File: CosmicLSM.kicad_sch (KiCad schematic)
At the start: 49 parts, among them J1 BAT, J2 JST GH, J3 USB_C_Receptacle_USB2.0, SW1 SW_SPDT, SW2 SW_SPST, U1 SMF05CT1G, U2 SMF05CT1G, U3 M3406, U4 IP2312, U5 LSM6DSV, U7 ESP32-C6-MINI-1/U

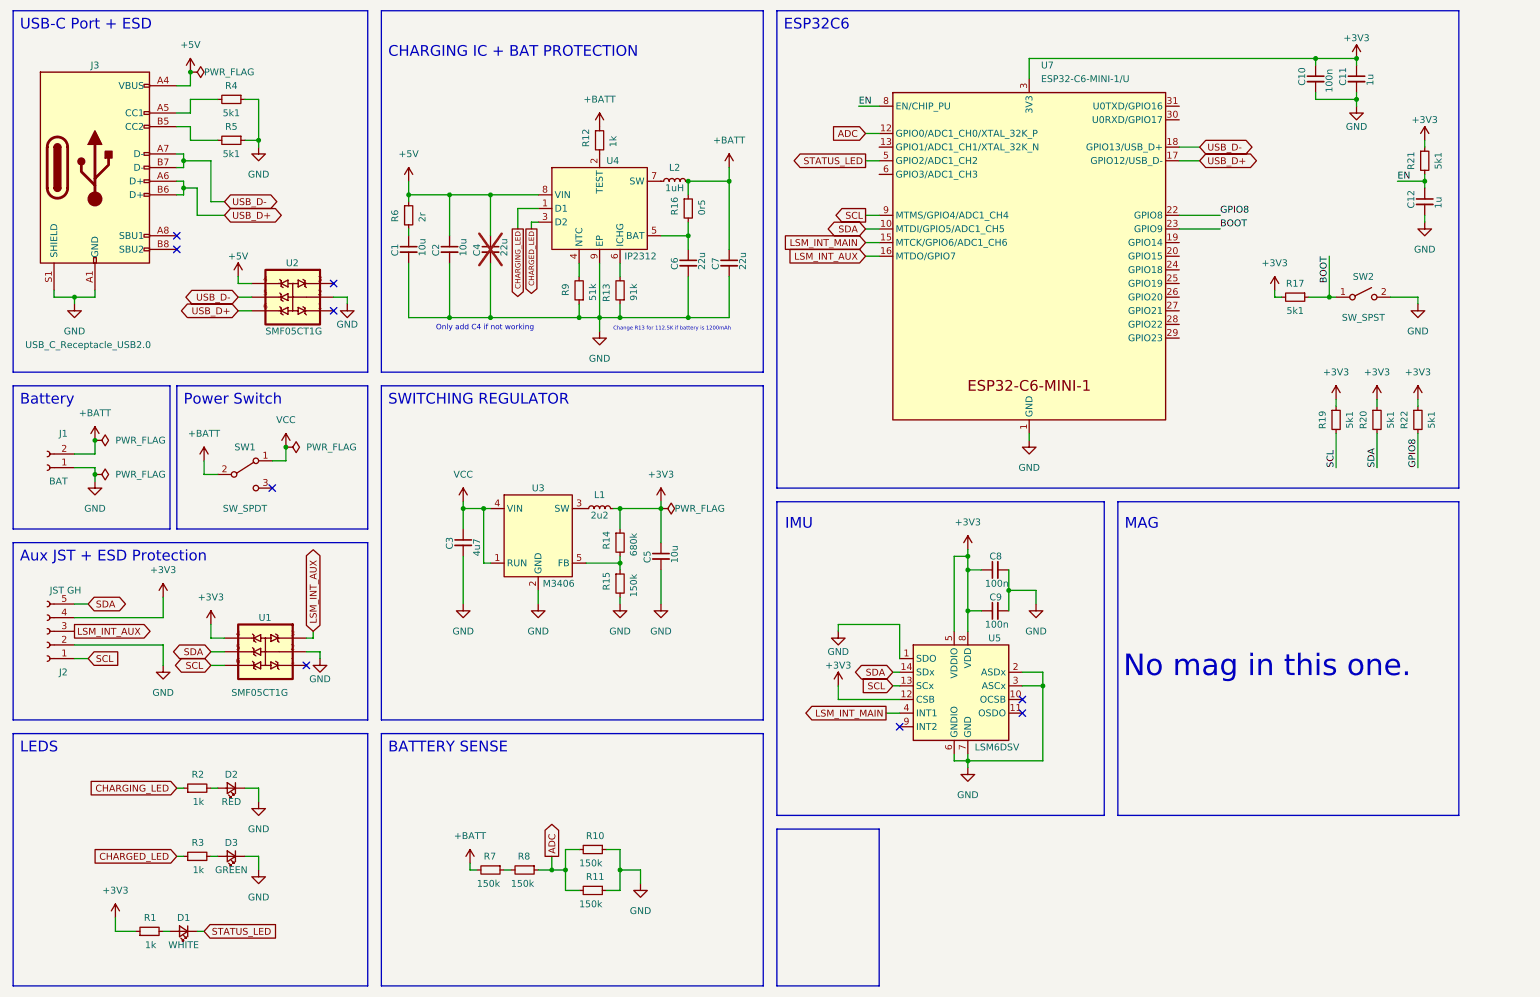
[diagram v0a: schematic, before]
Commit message: new data
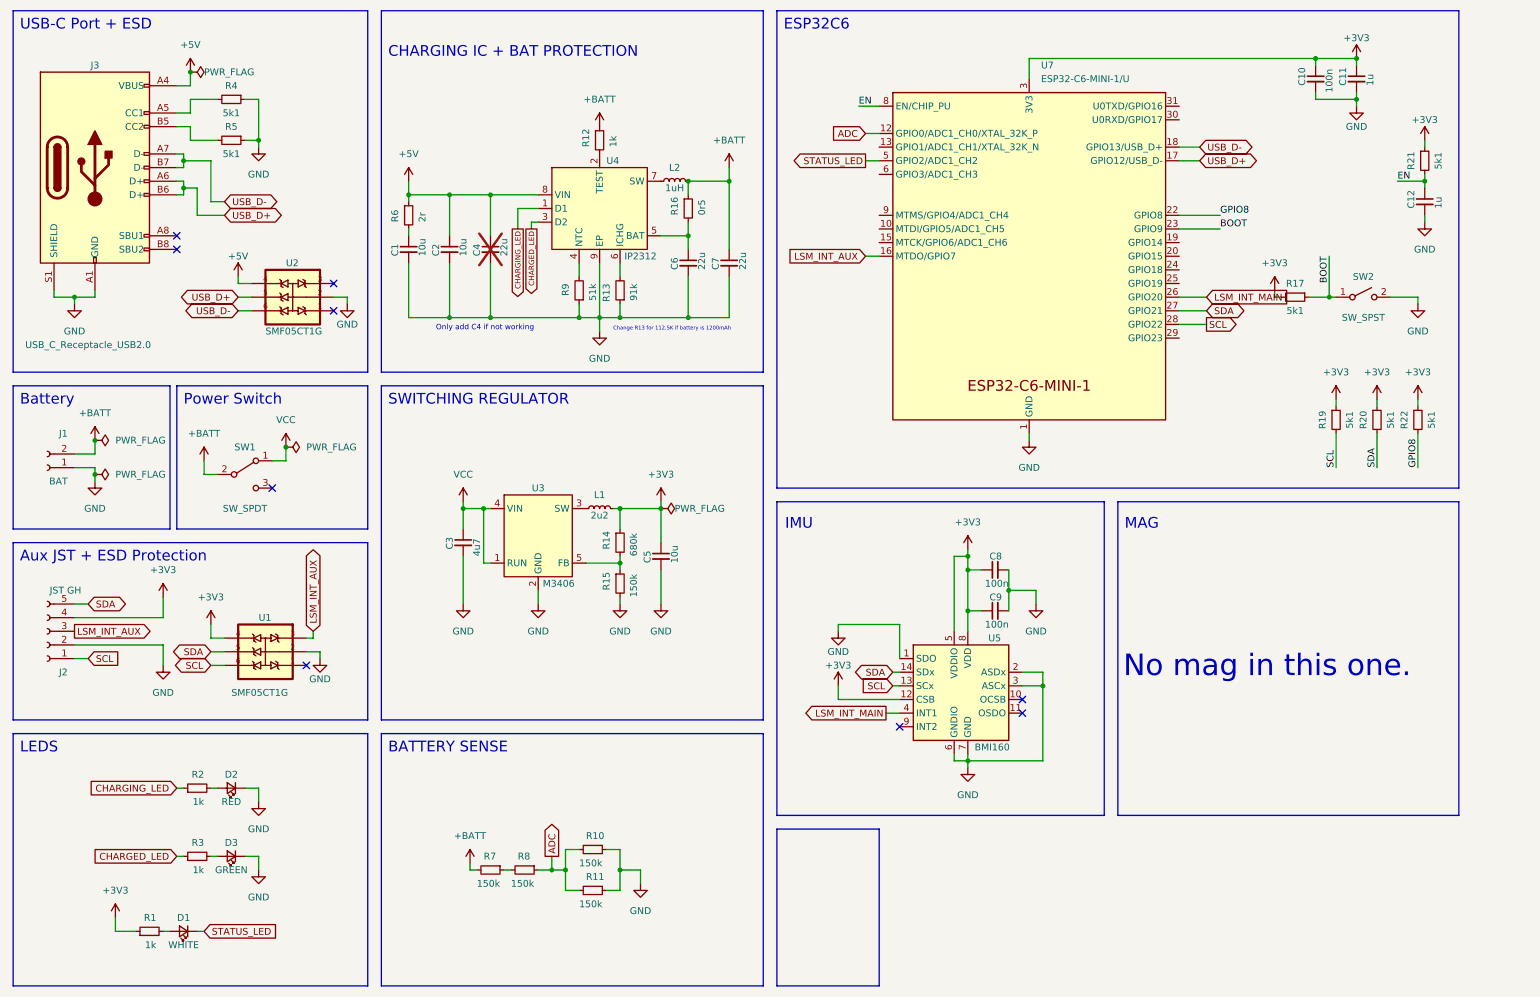
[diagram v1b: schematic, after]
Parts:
- U5: value LSM6DSV -> BMI160
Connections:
- net LSM_INT_MAIN: now also U7.26 (GPIO20); no longer U7.15 (MTCK/GPIO6/ADC1_CH6)
- net SCL: now also U7.28 (GPIO22); no longer U7.9 (MTMS/GPIO4/ADC1_CH4)
- net SDA: now also U7.27 (GPIO21); no longer U7.10 (MTDI/GPIO5/ADC1_CH5)
- net USB_D+: now also U2.5; no longer U2.6
- net USB_D-: now also U2.6; no longer U2.5
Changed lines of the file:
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@@
 	(wire
 		(pts
-			(xy 172.72 54.61) (xy 175.26 54.61)
-		)
-		(stroke
-			(width 0)
-			(type default)
-		)
-	)
-	(wire
-		(pts
 			(xy 73.66 67.31) (xy 76.2 67.31)
 		)
@@
 	(wire
 		(pts
-			(xy 45.72 41.91) (xy 45.72 40.64)
+			(xy 231.14 67.31) (xy 236.22 67.31)
 		)
 		(stroke
@@
 	(wire
 		(pts
-			(xy 172.72 57.15) (xy 175.26 57.15)
+			(xy 231.14 72.39) (xy 236.22 72.39)
+		)
+		(stroke
+			(width 0)
+			(type default)
+		)
+	)
+	(wire
+		(pts
+			(xy 45.72 41.91) (xy 45.72 40.64)
 		)
 		(stroke
@@
 	(wire
 		(pts
-			(xy 172.72 52.07) (xy 175.26 52.07)
-		)
-		(stroke
-			(width 0)
-			(type default)
-		)
-	)
-	(wire
-		(pts
 			(xy 116.84 173.99) (xy 116.84 170.18)
 		)
@@
 	(wire
 		(pts
+			(xy 231.14 69.85) (xy 236.22 69.85)
+		)
+		(stroke
+			(width 0)
+			(type default)
+		)
+	)
+	(wire
+		(pts
 			(xy 124.46 170.18) (xy 127 170.18)
 		)
@@
 		)
 	)
-	(global_label "USB_D-"
+	(global_label "USB_D+"
 		(shape bidirectional)
 		(at 55.88 67.31 180)
@@
 		)
 	)
-	(global_label "USB_D+"
+	(global_label "USB_D-"
 		(shape bidirectional)
 		(at 55.88 69.85 180)
@@
 	(global_label "SDA"
 		(shape bidirectional)
-		(at 172.72 54.61 180)
+		(at 236.22 69.85 0)
 		(fields_autoplaced yes)
 		(effects
@@
 				(size 1.27 1.27)
 			)
-			(justify right)
+			(justify left)
 		)
 		(property "Intersheetrefs" "${INTERSHEET_REFS}"
-			(at 165.0554 54.61 0)
+			(at 243.8846 69.85 0)
 			(effects
 				(font
 					(size 1.27 1.27)
 				)
-				(justify right)
+				(justify left)
 				(hide yes)
 			)
@@
 	(global_label "LSM_INT_MAIN"
 		(shape input)
-		(at 172.72 57.15 180)
+		(at 236.22 67.31 0)
 		(fields_autoplaced yes)
 		(effects
@@
 				(size 1.27 1.27)
 			)
-			(justify right)
+			(justify left)
 		)
 		(property "Intersheetrefs" "${INTERSHEET_REFS}"
-			(at 156.7324 57.15 0)
+			(at 252.2076 67.31 0)
 			(effects
 				(font
 					(size 1.27 1.27)
 				)
-				(justify right)
+				(justify left)
 				(hide yes)
 			)
@@
 	(global_label "SCL"
 		(shape output)
-		(at 172.72 52.07 180)
+		(at 236.22 72.39 0)
 		(fields_autoplaced yes)
 		(effects
@@
 				(size 1.27 1.27)
 			)
-			(justify right)
+			(justify left)
 		)
 		(property "Intersheetrefs" "${INTERSHEET_REFS}"
-			(at 166.2272 52.07 0)
+			(at 242.7128 72.39 0)
 			(effects
 				(font
 					(size 1.27 1.27)
 				)
-				(justify right)
+				(justify left)
 				(hide yes)
 			)
@@
 			)
 		)
-		(property "Value" "LSM6DSV"
+		(property "Value" "BMI160"
 			(at 193.04 151.13 0)
 			(effects
